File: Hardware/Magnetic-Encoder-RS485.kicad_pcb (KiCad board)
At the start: 2 copper layers, 42 x 42 mm, 32 parts, among them J1 Conn_01x04, J2 Conn_01x04, U1 STM8S003F3P, U2 SP3485EN, U3 MT6816CT-ACD, U4 HT75R33-1A, Y1 X1E0000210119

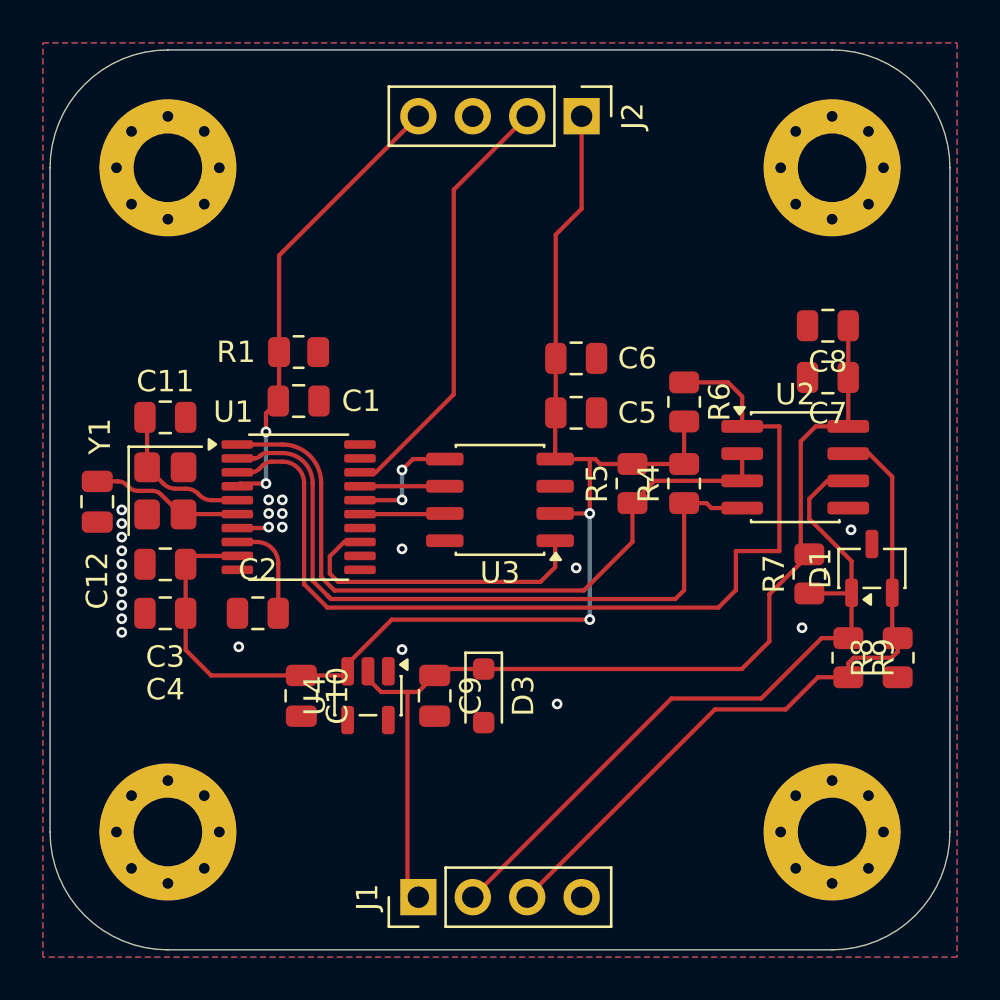
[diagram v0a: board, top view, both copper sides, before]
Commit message: Design is almost done
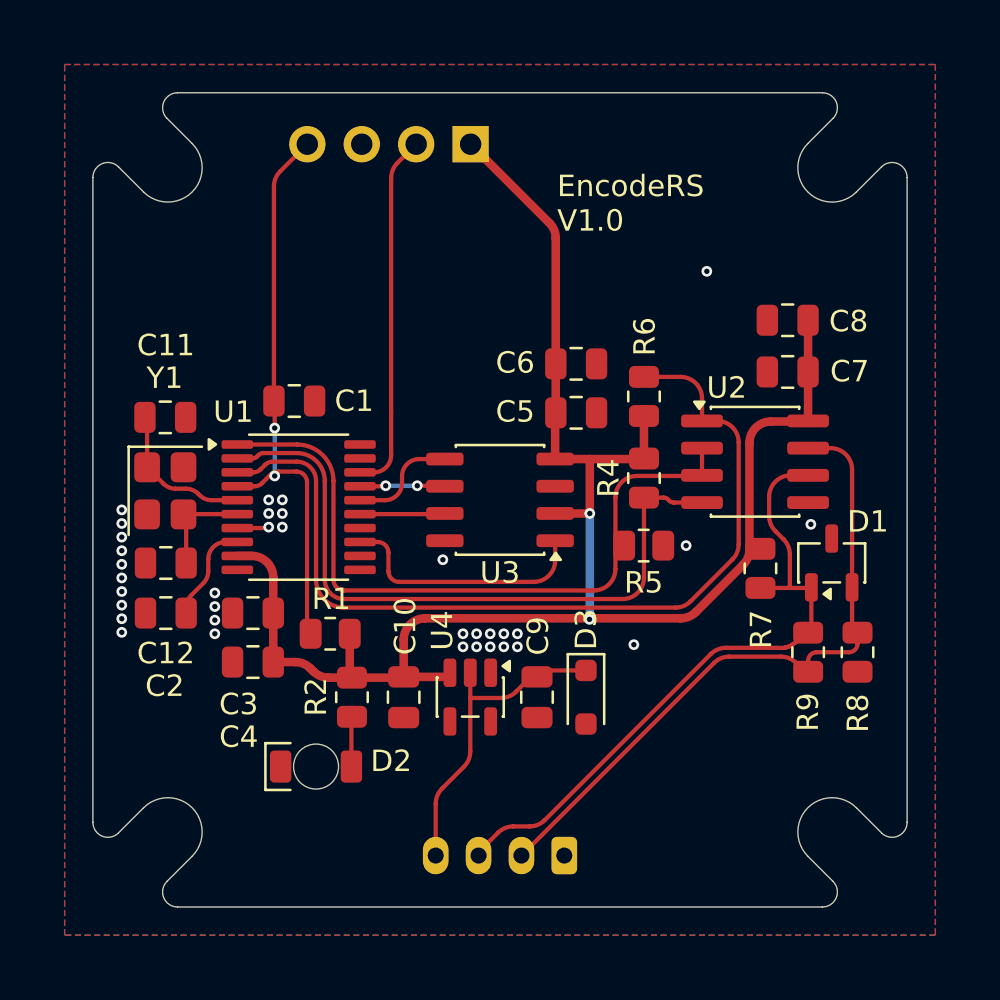
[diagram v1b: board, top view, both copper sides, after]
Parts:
- removed H1, H2, H3, H4: MountingHole_Pad, MountingHole:MountingHole_3.2mm_M3_Pad_Via
- added D2: LED, LED_SMD:LED_1206_3216Metric_ReverseMount_Hole1.8x2.4mm, F.Cu at (32.8, 53.3)
- added G***: LOGO, LOGO, B.Cu at (41.4, 42.1)
- added R2: 100, Resistor_SMD:R_0805_2012Metric, F.Cu at (34.5, 50.1)
- J1: footprint Connector_PinHeader_2.54mm:PinHeader_1x04_P2.54mm_Vertical -> Connector_JST:JST_PH_S4B-PH-K_1x04_P2.00mm_Horizontal; moved to B.Cu
- J2: moved to B.Cu
- moved R1 13.2 mm to (33.5, 47.1)
- moved J1 7.08 mm to (44.4, 57.5), turned to 180 degrees
- moved J2 5.34 mm to (40.0, 24.3), turned to 90 degrees
- moved C9 4.78 mm to (43.1, 50.1)
- moved C10 4.78 mm to (36.9, 50.1)
- moved D3 4.78 mm to (45.4, 50.1)
- moved U4 4.78 mm to (40.0, 50.1)
- moved C3 4.68 mm to (29.8, 46.2)
- moved C4 4.68 mm to (29.8, 48.4)
- moved C2 4.29 mm to (25.8, 46.2)
- moved C12 4.29 mm to (25.8, 43.8), turned to 180 degrees
- moved R5 2.94 mm to (48.1, 43.0), turned to 180 degrees
- moved R7 2.30 mm to (53.5, 44.1)
- moved D1 1.89 mm to (56.9, 43.8)
- moved C7 1.89 mm to (54.8, 34.9)
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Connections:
- J1 pad 1: +5V -> GND
- J1 pad 2: /A -> /B
- J1 pad 3: /B -> /A
- J1 pad 4: GND -> +5V
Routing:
- net +5V: track 48.2 -> 16.0 mm
- net +3V3: track 60.9 -> 81.8 mm
- net /NRST: track 21.5 -> 27.2 mm
- net /SWIM: track 20.3 -> 16.8 mm
- net /RX: track 45.2 -> 42.0 mm
- net /A: track 34.1 -> 30.9 mm
- net /CSN: track 14.7 -> 12.0 mm
- net Net-(D2-A): track 0.00 -> 2.72 mm
- net Net-(U1-PA2): track 7.25 -> 4.95 mm
- net /TX: track 33.7 -> 31.9 mm
- net /B: track 33.2 -> 31.6 mm
- net /MOSI: track 5.57 -> 5.13 mm, vias 2 -> 0
- net /MISO: track 3.96 -> 3.93 mm, vias 0 -> 2
- net GND: vias 23 -> 35
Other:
- board size 42 x 42 mm -> 38 x 38 mm
- board text added: "EncodeRS V1.0"
